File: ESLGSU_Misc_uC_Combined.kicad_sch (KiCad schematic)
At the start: 6 parts, among them U57 CY8C9520A, U74 PCAL6524HEAZ

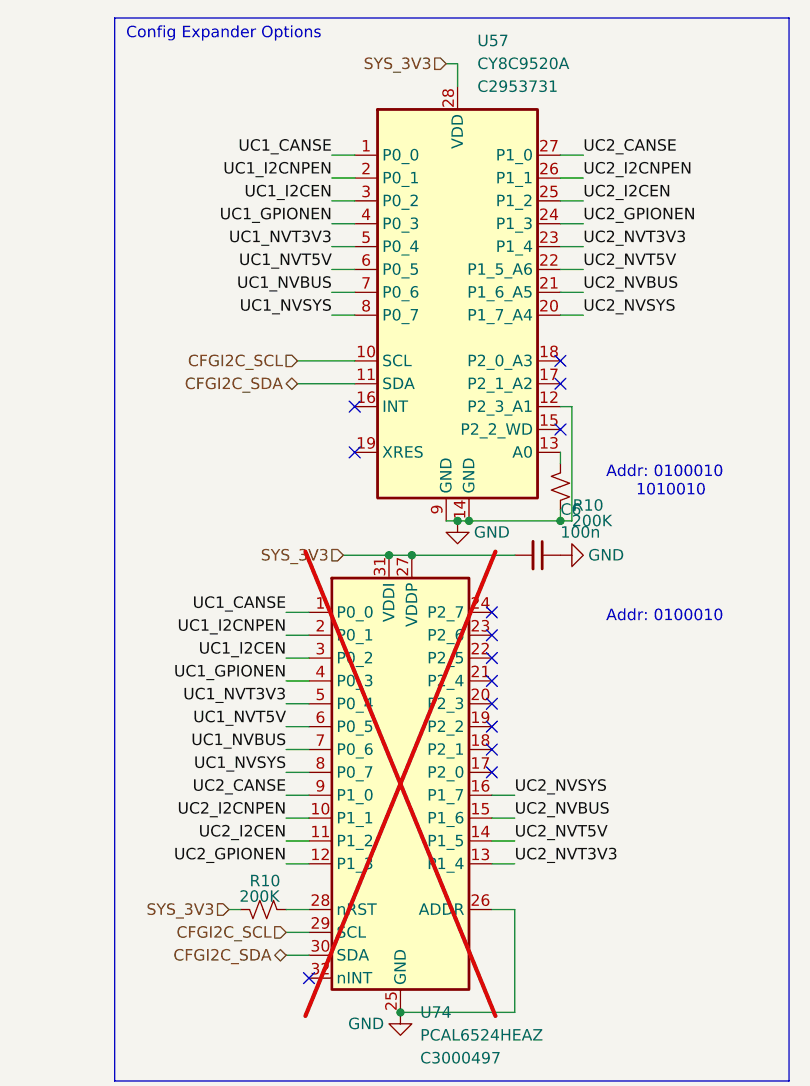
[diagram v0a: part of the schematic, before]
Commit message: Minimal version
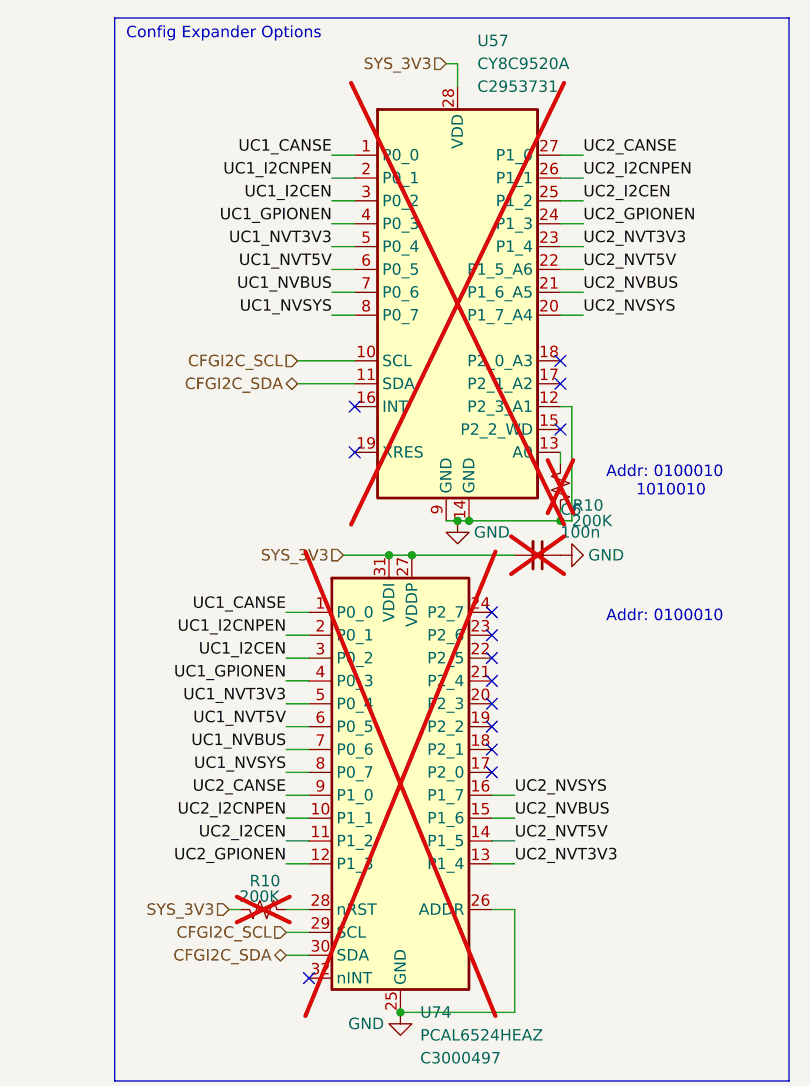
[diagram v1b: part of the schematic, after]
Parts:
- C6, R10, U57: JLCPCB BOM (none) -> 0; now not fitted; now left out of the parts list
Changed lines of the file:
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@@
   )
   (symbol (lib_id "Device:R_Small_US") (at 214.63 82.55 0) (mirror x) (unit 1)
-    (in_bom yes) (on_board yes) (dnp no)
+    (in_bom no) (on_board yes) (dnp yes)
     (property "Reference" "R10" (at 215.9914 84.6363 0)
       (effects (font (size 1.27 1.27)) (justify left))
@@
     )
     (property "LCSC Part" "C25764" (at 211.9986 88.0837 0)
+      (effects (font (size 1.27 1.27)) hide)
+    )
+    (property "JLCPCB BOM" "0" (at 214.63 82.55 0)
       (effects (font (size 1.27 1.27)) hide)
     )
@@
   )
   (symbol (lib_id "Device:C_Small") (at 212.09 90.17 270) (unit 1)
-    (in_bom yes) (on_board yes) (dnp no)
+    (in_bom no) (on_board yes) (dnp yes)
     (property "Reference" "C6" (at 214.63 85.09 90)
       (effects (font (size 1.27 1.27)) (justify left))
@@
     )
     (property "LCSC Part" "C307331" (at 214.63 87.63 90)
+      (effects (font (size 1.27 1.27)) hide)
+    )
+    (property "JLCPCB BOM" "0" (at 212.09 90.17 90)
       (effects (font (size 1.27 1.27)) hide)
     )
@@
   )
   (symbol (lib_id "Device:R_Small_US") (at 181.61 129.54 90) (mirror x) (unit 1)
-    (in_bom yes) (on_board yes) (dnp no)
+    (in_bom no) (on_board yes) (dnp yes)
     (property "Reference" "R10" (at 183.515 126.365 90)
       (effects (font (size 1.27 1.27)) (justify left))
@@
     )
     (property "LCSC Part" "C25764" (at 176.0763 126.9086 0)
+      (effects (font (size 1.27 1.27)) hide)
+    )
+    (property "JLCPCB BOM" "0" (at 181.61 129.54 90)
       (effects (font (size 1.27 1.27)) hide)
     )
@@
   )
   (symbol (lib_id "ESLGSU_Parts_Lib:CY8C9520A") (at 203.2 54.61 0) (unit 1)
-    (in_bom yes) (on_board yes) (dnp no) (fields_autoplaced)
+    (in_bom no) (on_board yes) (dnp yes) (fields_autoplaced)
     (property "Reference" "U57" (at 205.3941 33.02 0)
       (effects (font (size 1.27 1.27)) (justify left))
@@
       (effects (font (size 1.27 1.27)) (justify left))
     )
+    (property "JLCPCB BOM" "0" (at 203.2 54.61 0)
+      (effects (font (size 1.27 1.27)) hide)
+    )
     (pin "10")
